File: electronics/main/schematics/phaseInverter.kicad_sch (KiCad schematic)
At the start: 1 part

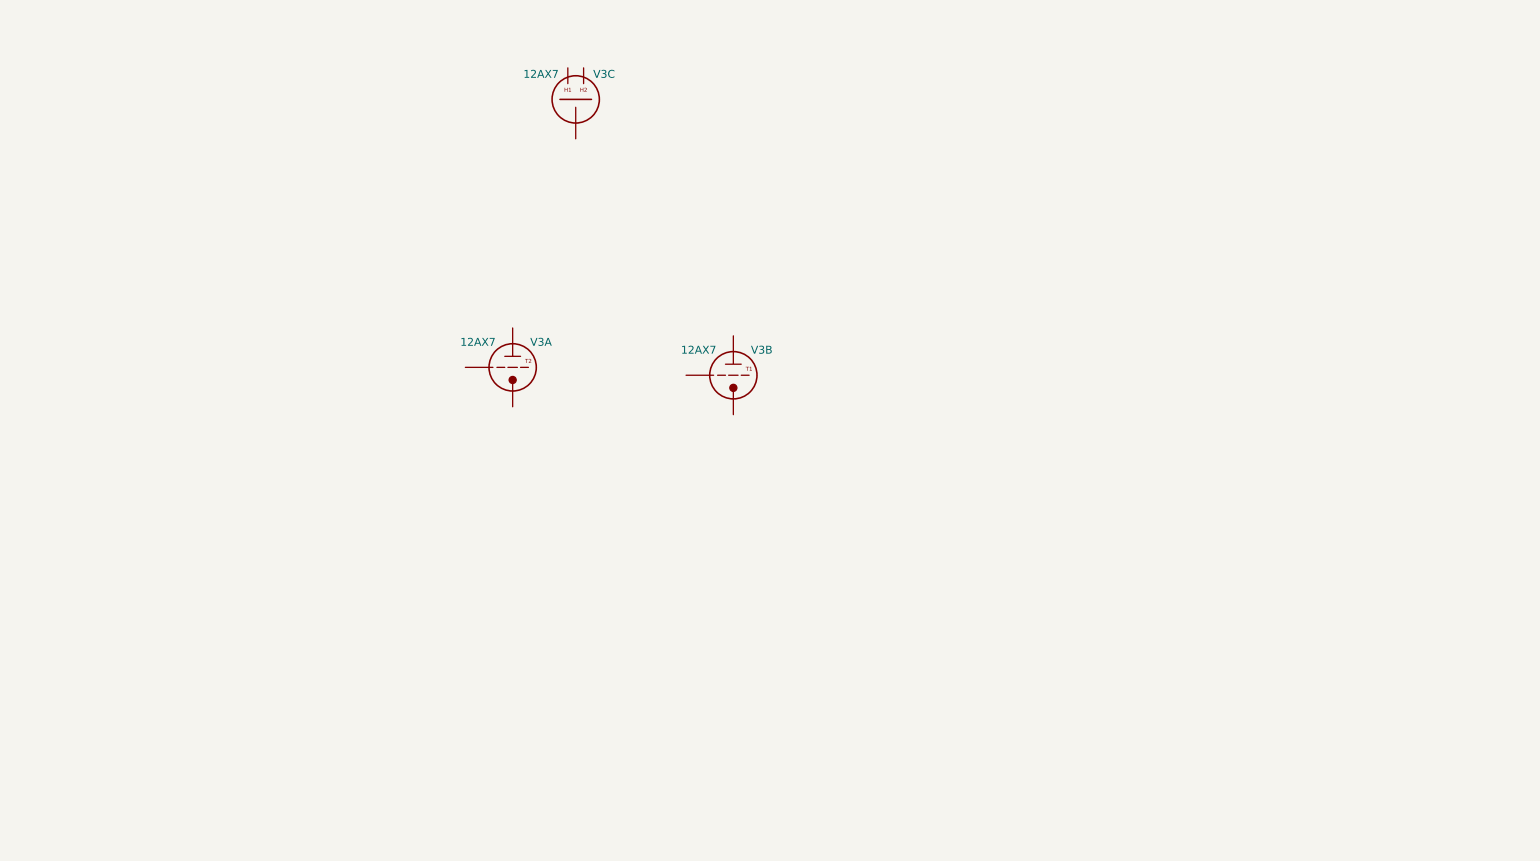
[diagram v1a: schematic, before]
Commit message: PI stage ready
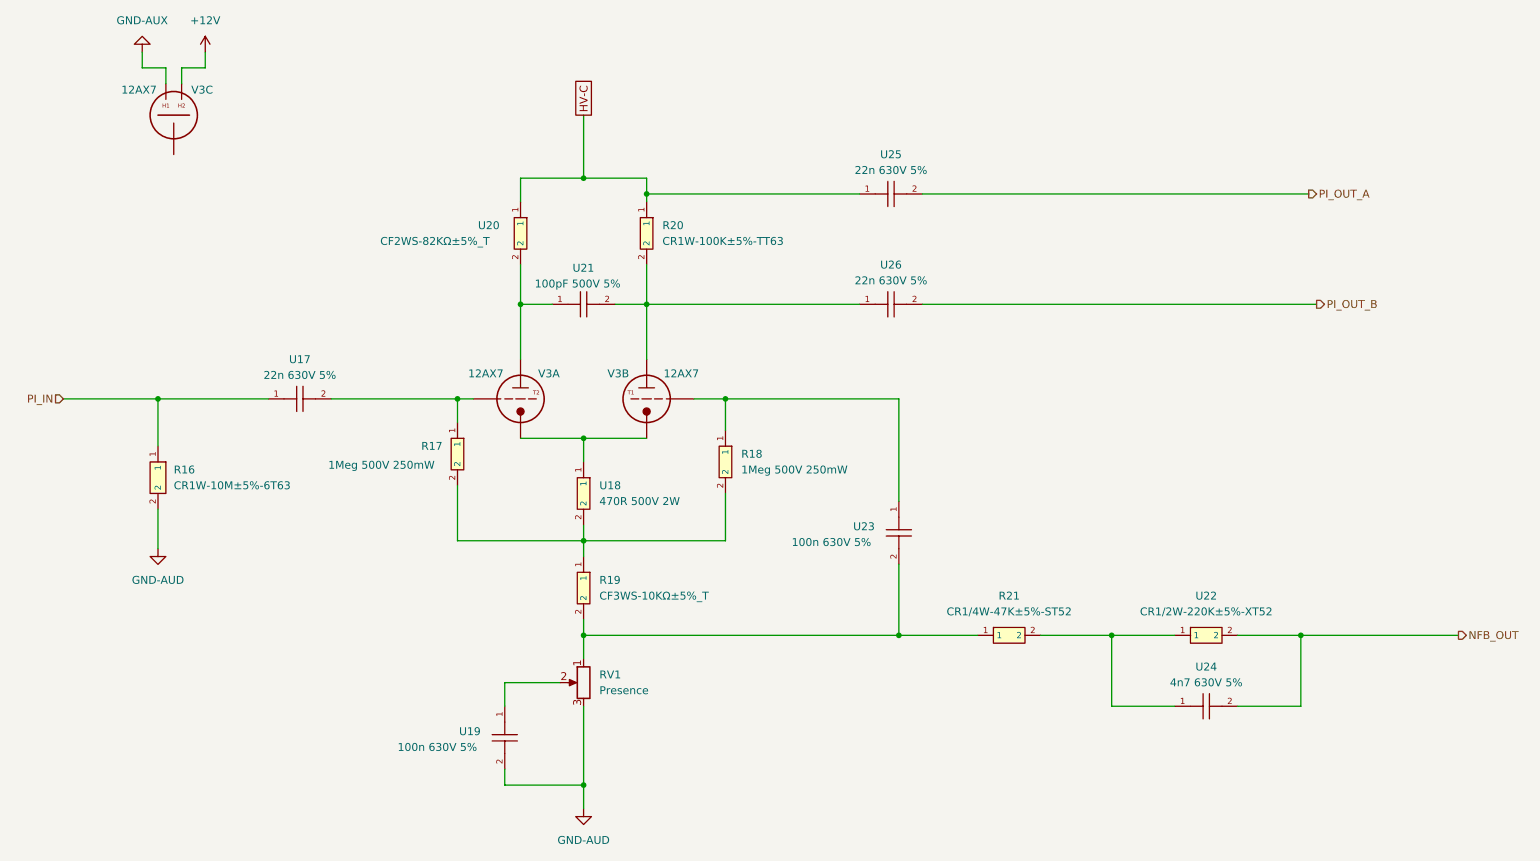
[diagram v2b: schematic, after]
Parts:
- added R16: CR1W-10M±5%-6T63, footprints:RES-TH_BD4.5-L11.0-P15.00-D0.7, symbol jlcpcb:CR1W-10M±5%-6T63
- added R17, R18: 1Meg 500V 250mW, footprints:RES-TH_BD2.4-L6.3-P10.30-D0.6, symbol jlcpcb:CFR-25JT-52-1M
- added R19: CF3WS-10KΩ±5%_T, footprints:RES-TH_BD5.5-L15.0-P19.00-D0.8, symbol jlcpcb:CF3WS-10KΩ±5%_T
- added R20: CR1W-100K±5%-TT63, footprints:RES-TH_BD4.5-L11.0-P15.00-D0.7, symbol jlcpcb:CR1W-100K±5%-TT63
- added R21: CR1/4W-47K±5%-ST52, footprints:RES-TH_BD2.7-L6.2-P10.20-D0.4, symbol jlcpcb:CR1/4W-47K±5%-ST52
- added RV1: Presence, wb50_footprints:WB50_Pot_Omeg_PC20BU_P5.00mm, symbol Device:R_Potentiometer
- added U17, U25, U26: 22n 630V 5%, wb50_footprints:MUSTARD_CAP_D8.5_L20.5_P25.5, symbol wb50_symbols:YellowCap_4n7_630V
- added U18: 470R 500V 2W, footprints:RES-TH_BD5.0-L15.5-P19.50-D0.7, symbol jlcpcb:CFR02SJ0471A10
- added U19, U23: 100n 630V 5%, wb50_footprints:MUSTARD_CAP_D10_L32_P40.4, symbol wb50_symbols:YellowCap_100n_630V
- added U20: CF2WS-82KΩ±5%_T, footprints:RES-TH_BD4.0-L11.5-P15.50-D0.7, symbol jlcpcb:CF2WS-82KΩ±5%_T
- added U21: 100pF 500V 5%, wb50_footprints:MICA_CAP_L15.5_W3.6_P8.7, symbol wb50_symbols:MicaCap_500pf_500V
- added U22: CR1/2W-220K±5%-XT52, footprints:RES-TH_BD3.5-L9.0-P13.00-D0.5, symbol jlcpcb:CR1/2W-220K±5%-XT52
- added U24: 4n7 630V 5%, wb50_footprints:MUSTARD_CAP_D8.5_L20.5_P25.5, symbol wb50_symbols:YellowCap_4n7_630V
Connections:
- net +12V: now reaches V3.4 (H1)
- net GND-AUX: now reaches V3.5 (H2)
- net at V3.1 (A/P): now also U20.2, U21.1
- net at V3.2 (G): now also R17.1, U17.2
- net at V3.3 (C/K): now also V3.8 (C/K), U18.1
- net at V3.6 (A/P): now also R20.2, U21.2, U26.1
- net at V3.7 (G): now also R18.1, U23.1
- new net: R21.2, U22.1, U24.1
- new net: R19.2, R21.1, RV1.1, U23.2
- new net: RV1.2, U19.1
- new net: R17.2, R18.2, R19.1, U18.2
- new net GND-AUD: R16.2, RV1.3, U19.2
- new net HV-C: R20.1, U20.1, U25.1
- new net NFB_OUT: U22.2, U24.2
- new net PI_IN: R16.1, U17.1
- new net PI_OUT_A: U25.2
- new net PI_OUT_B: U26.2
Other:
- moved on the sheet: V3A, V3B, V3C
